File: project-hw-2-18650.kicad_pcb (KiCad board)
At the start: 2 copper layers, 98 x 44 mm, 15 parts, among them J1 2060-452_998-404, U1 TPS62933

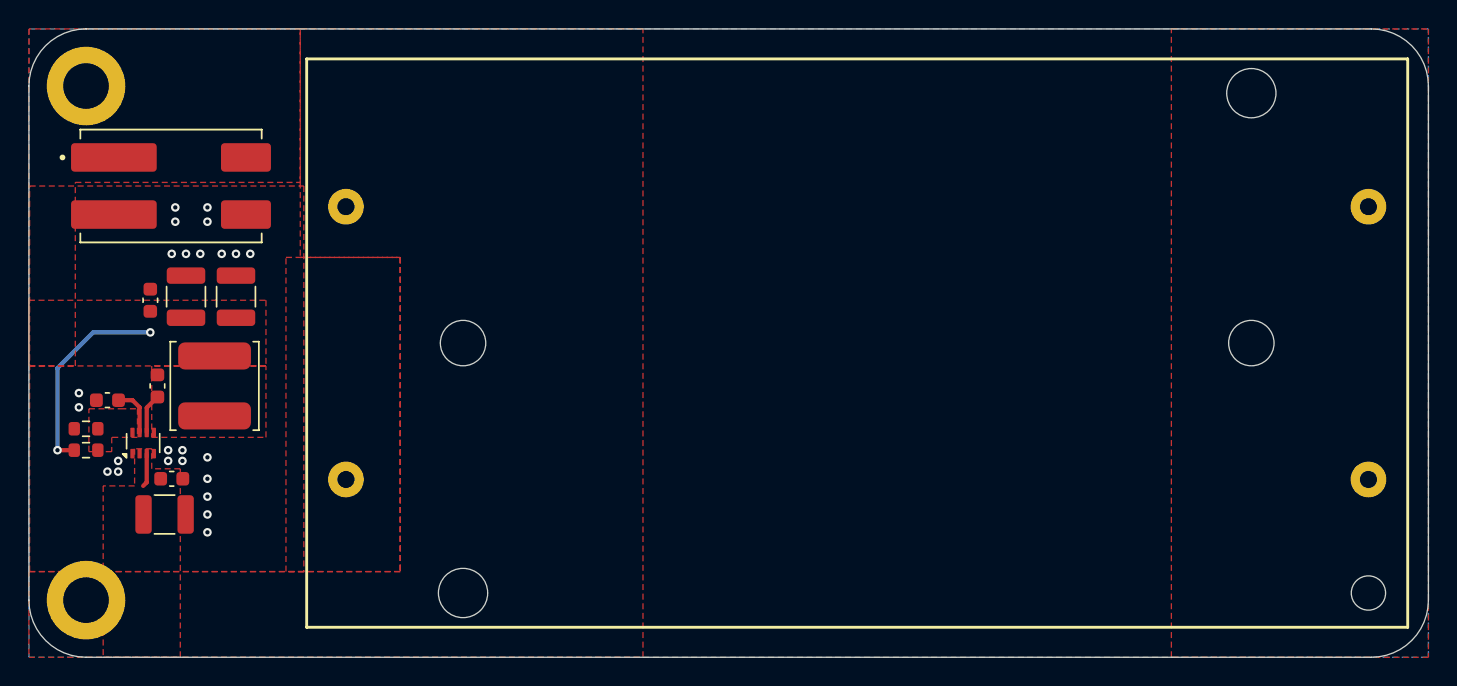
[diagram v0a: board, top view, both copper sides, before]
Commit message: pcb: routing v2
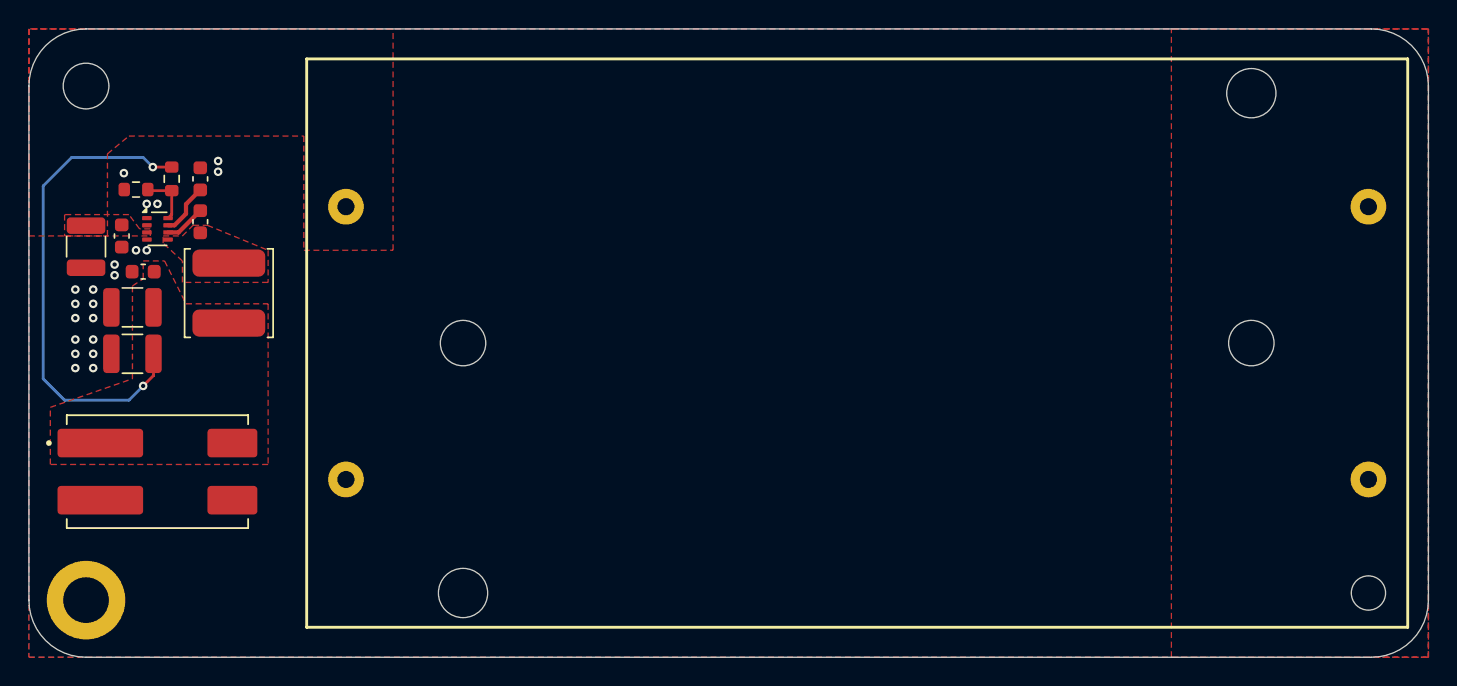
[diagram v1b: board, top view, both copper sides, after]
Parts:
- H1: value MountingHole_Pad -> MountingHole; footprint MountingHole:MountingHole_3.2mm_M3_ISO14580_Pad -> MountingHole:MountingHole_3.2mm_M3_ISO14580
- moved J1 20.0 mm to (27.0, 47.0)
- moved R1 19.9 mm to (28.0, 26.5), turned to -90 degrees
- moved C1 19.5 mm to (22.0, 31.2), turned to -90 degrees
- moved C2 17.4 mm to (24.5, 30.5), turned to -90 degrees
- moved R2 17.1 mm to (25.5, 27.2)
- moved C3 16.8 mm to (30.0, 26.5), turned to 90 degrees
- moved U1 15.0 mm to (27.0, 30.0), turned to 0 degrees
- moved C4 11.9 mm to (30.0, 29.5), turned to -90 degrees
- moved C6 8.28 mm to (25.2, 38.8), turned to 180 degrees
- moved L1 6.58 mm to (32.0, 34.5), turned to -90 degrees
- moved C7 3.82 mm to (25.2, 35.5), turned to 180 degrees
- moved C5 2.06 mm to (26.0, 33.0), turned to 180 degrees
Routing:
- net /TPS6293x Converter/Vout: track 14.5 -> 34.2 mm
- net Net-(U1-FB): track 0.00 -> 3.74 mm
- net +BATT: track 2.36 -> 0.00 mm
- net GND: vias 24 -> 21
- removed copper zone on F.Cu, net Net-(U1-FB)
